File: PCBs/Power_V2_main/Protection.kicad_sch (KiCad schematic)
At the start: 27 parts, among them J10 TYPE-C-31-M-12, J12 Conn_01x02, J18 YK4420203000G, J2 Conn_01x02, J3 Conn_01x02, U4 178.6164.0001, U5 TVS3300DRV, U9 AMS1117-3.3

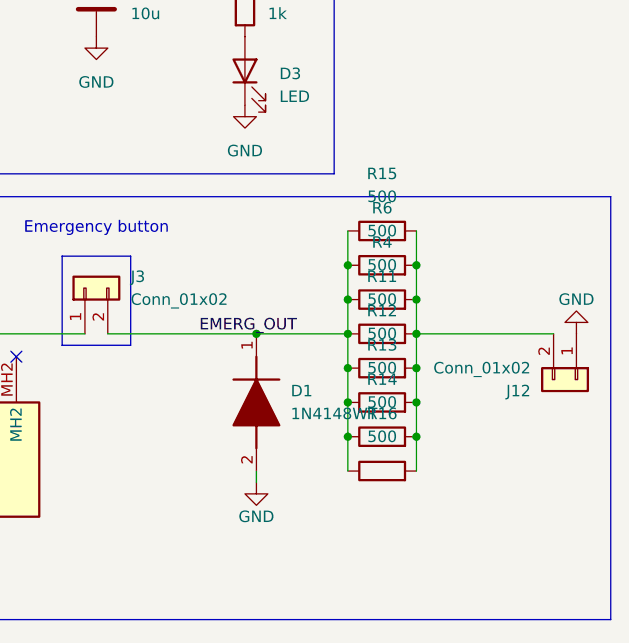
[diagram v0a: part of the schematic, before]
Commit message: follow up changes from meeting
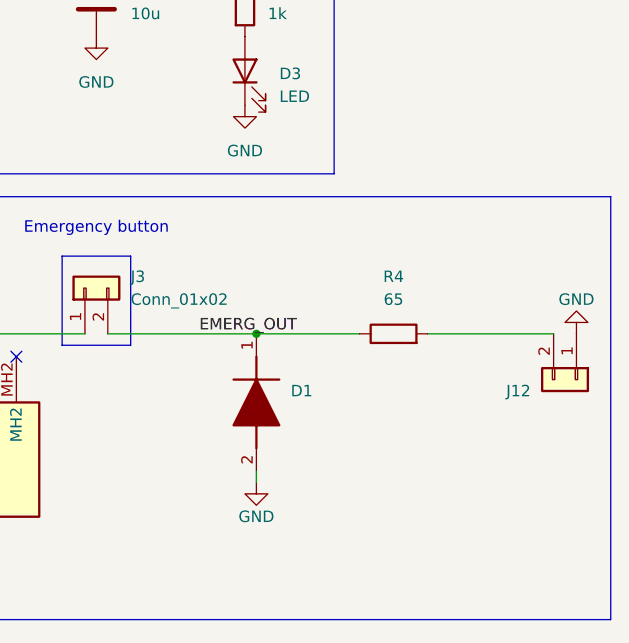
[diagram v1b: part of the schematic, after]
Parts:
- removed R11, R12, R13, R14, R15, R16, R6: 500, Resistor_SMD:R_0805_2012Metric, symbol Device:R
- R4: value 500 -> 65; footprint Resistor_SMD:R_0805_2012Metric -> Resistor_THT:R_Axial_DIN0414_L11.9mm_D4.5mm_P15.24mm_Horizontal
